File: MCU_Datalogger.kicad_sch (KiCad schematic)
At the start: 25 parts, among them U1 24LC1025, U2 24LC1025, U3 DS1337S_, U4 ATMEGA328P-AN, Y1 16 MHz, Y2 32.768 KHz

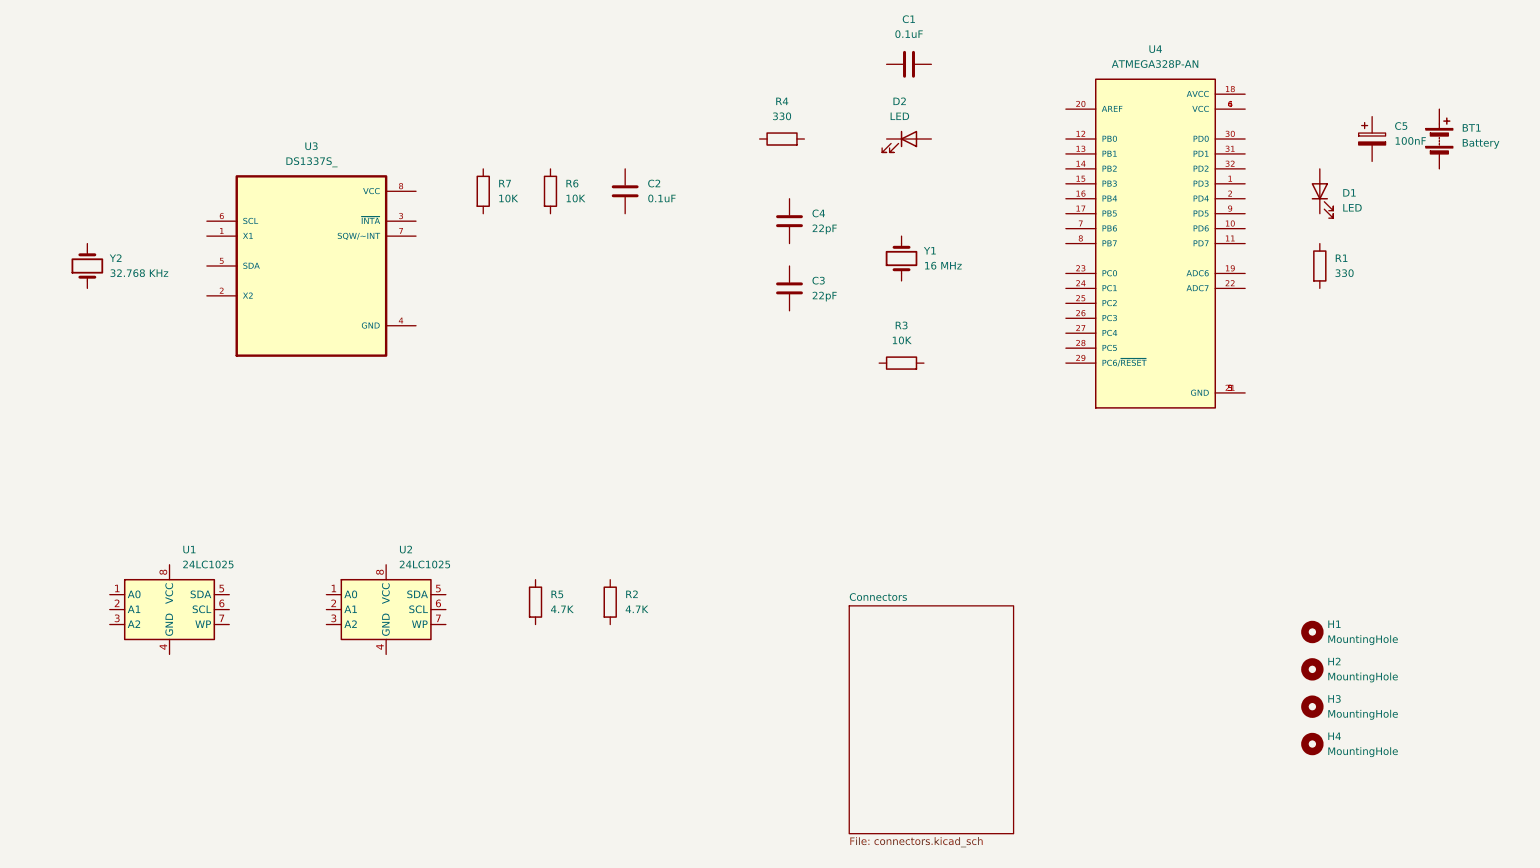
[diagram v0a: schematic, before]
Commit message: Finished Wiring of Main Sheet.
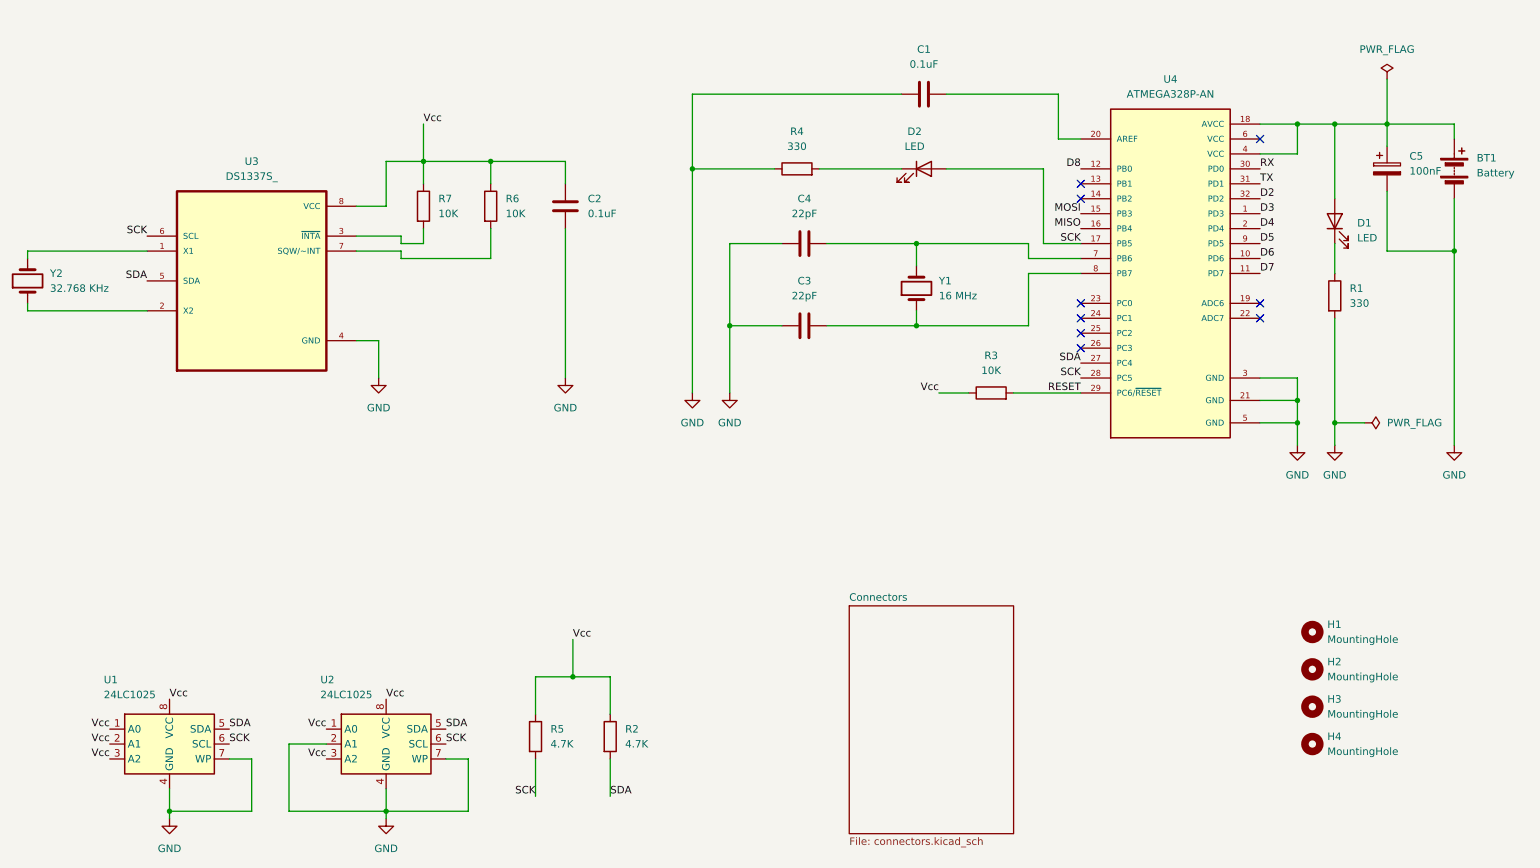
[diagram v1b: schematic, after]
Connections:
- net at Y1.1: now also C3.2, U4.8 (PB7)
- net at Y1.2: now also C4.2, U4.7 (PB6)
- net Vcc: now reaches C2.1
- net Vcc: now also R2.1, R3.1, R5.1, R6.1, R7.1, U1.1 (A0), U1.2 (A1), U1.3 (A2), U1.8 (VCC), U2.1 (A0), U2.3 (A2), U2.8 (VCC), U3.8 (VCC)
- net GND: now reaches C2.2
- net GND: now also BT1.2 (-), C1.1, C3.1, C4.1, C5.2, R1.2, R4.1, U1.4 (GND), U1.7 (WP), U2.2 (A1), U2.4 (GND), U2.7 (WP), U3.4 (GND), U4.21 (GND), U4.3 (GND), U4.5 (GND)
- net at Y2.1: now also U3.2 (X2)
- net at Y2.2: now also U3.1 (X1)
- net at D2.1 (K): now also R4.2
- net SCK: now reaches D2.2 (A)
- net SCK: now also R5.2, U1.6 (SCL), U2.6 (SCL), U3.6 (SCL), U4.17 (PB5), U4.28 (PC5)
- net D3: now reaches U4.1 (PD3)
- net D6: now reaches U4.10 (PD6)
- net D7: now reaches U4.11 (PD7)
- net D8: now reaches U4.12 (PB0)
- net MOSI: now reaches U4.15 (PB3)
- net MISO: now reaches U4.16 (PB4)
- net at U4.18 (AVCC): now also BT1.1 (+), C5.1, D1.2 (A), U4.4 (VCC)
- net D4: now reaches U4.2 (PD4)
- net at U4.20 (AREF): now also C1.2
- net SDA: now reaches U4.27 (PC4)
- net SDA: now also R2.2, U1.5 (SDA), U2.5 (SDA), U3.5 (SDA)
- net RESET: now reaches U4.29 (PC6/~{RESET})
- net RESET: now also R3.2
- net RX: now reaches U4.30 (PD0)
- net TX: now reaches U4.31 (PD1)
- net D2: now reaches U4.32 (PD2)
- net at U4.6 (VCC): no longer U4.4 (VCC)
- net D5: now reaches U4.9 (PD5)
- net at R1.1: now also D1.1 (K)
- net at U3.3 (~{INTA}): now also R7.2
- net at U3.7 (SQW/~INT): now also R6.2
- no-connect marks 0 -> 9
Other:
- moved on the sheet: BT1, C1, C2, C3, C4, C5, D1, D2, R1, R2, R3, R4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
